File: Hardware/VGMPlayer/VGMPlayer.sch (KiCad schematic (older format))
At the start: 91 parts, among them J1 USB_B_Mini, Q1 9013, Q2 S8550, SW1 Mode, SW2 NEXT, SW3 PREV, SW4 SELECT, SW5 PWR, U1 STM32F103XX, U10 LTC6903, U11 HC-06, U13 YM3012, U14 LM324, U18 OLED_128_64_I2C, U19 ESP8266Module, U2 SDCardModule, U3 LM386, U4 LM386, U5 YM2151, U6 AUDIOJACK-VGM, U7 YM2612, U8 SN76489, U9 LTC6903

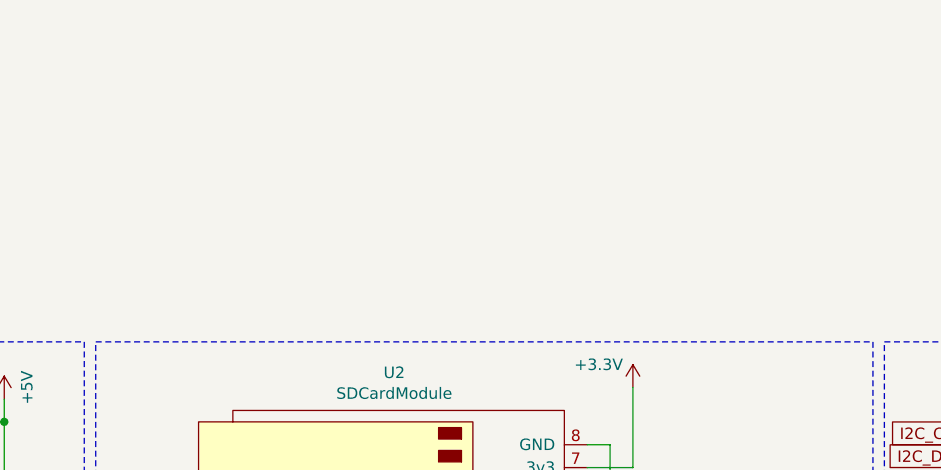
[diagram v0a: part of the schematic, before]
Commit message: 1
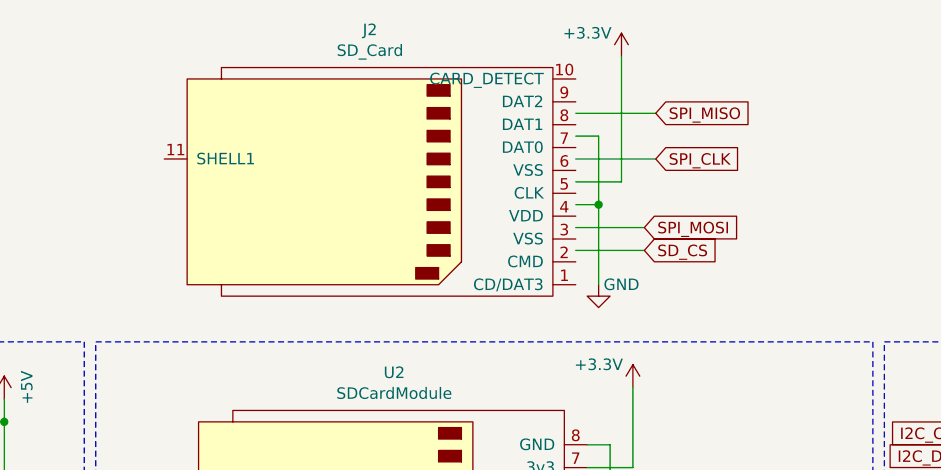
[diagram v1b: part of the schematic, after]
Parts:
- added J2: SD_Card, Connector_Card:SD_TE_2041021, symbol VGMPlayer-rescue:SD_Card
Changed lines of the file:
@@
 	0    1    1    0
 $EndComp
+$Comp
+L VGMPlayer-rescue:SD_Card J2
+U 1 1 5C3FE198
+P 16400 -150
+F 0 "J2" H 16400 -815 50  0000 C CNN
+F 1 "SD_Card" H 16400 -724 50  0000 C CNN
+F 2 "Connector_Card:SD_TE_2041021" H 16400 -150 50  0001 C CNN
+F 3 "http://portal.fciconnect.com/Comergent//fci/drawing/10067847.pdf" H 16400 -150 50  0001 C CNN
+	1    16400 -150
+	-1   0    0    1
+$EndComp
+Text GLabel 17650 -450 2    50   Input ~ 0
+SPI_MISO
+Text GLabel 17600 50   2    50   Input ~ 0
+SPI_MOSI
+Text GLabel 17650 -250 2    50   Input ~ 0
+SPI_CLK
+Text GLabel 17600 150  2    50   Input ~ 0
+SD_CS
+Wire Wire Line
+	17600 150  17300 150
+Wire Wire Line
+	17600 50   17300 50
+Wire Wire Line
+	17650 -450 17300 -450
+Wire Wire Line
+	17650 -250 17300 -250
+Wire Wire Line
+	17300 -350 17400 -350
+Wire Wire Line
+	17400 -350 17400 -50
+Wire Wire Line
+	17400 -50  17300 -50
+$Comp
+L power:GND #PWR0101
+U 1 1 5C6ABA25
+P 17400 300
+F 0 "#PWR0101" H 17400 50  50  0001 C CNN
+F 1 "GND" H 17500 300 50  0000 C CNN
+F 2 "" H 17400 300 50  0001 C CNN
+F 3 "" H 17400 300 50  0001 C CNN
+	1    17400 300
+	1    0    0    -1
+$EndComp
+Wire Wire Line
+	17400 -50  17400 300
+Connection ~ 17400 -50
+$Comp
+L power:+3.3V #PWR0102
+U 1 1 5C71FFAB
+P 17500 -700
+F 0 "#PWR0102" H 17500 -850 50  0001 C CNN
+F 1 "+3.3V" H 17350 -600 50  0000 C CNN
+F 2 "" H 17500 -700 50  0001 C CNN
+F 3 "" H 17500 -700 50  0001 C CNN
+	1    17500 -700
+	1    0    0    -1
+$EndComp
+Wire Wire Line
+	17500 -150 17300 -150
+Wire Wire Line
+	17500 -700 17500 -150
 $EndSCHEMATC
